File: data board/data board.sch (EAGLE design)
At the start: 41 parts, among them IC1 93LC56B, IC2 FT232HQ, U1 CJT1117-5.0-SOT223, X3 HUSB238, X6 USBC, Y1 12MHz

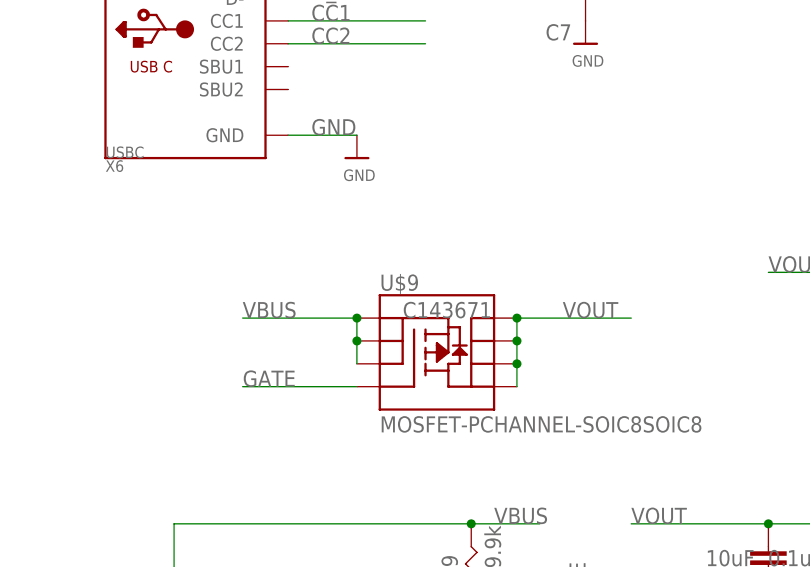
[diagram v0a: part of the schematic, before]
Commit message: v1.1
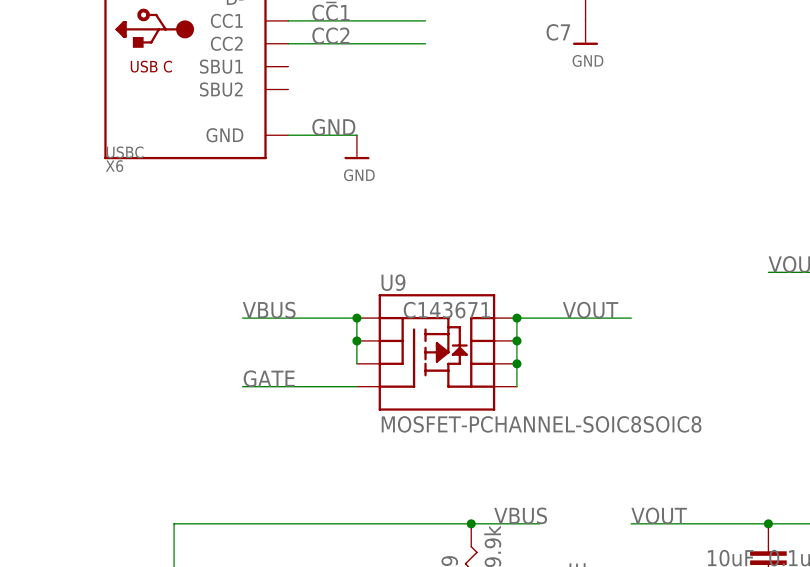
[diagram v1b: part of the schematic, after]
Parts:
- U1: LCSC (none) -> C89273
- renumbered U$9 to U9
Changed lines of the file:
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@@
 <part name="U$3" library="microbuilder" deviceset="GND" device=""/>
 <part name="JP3" library="microbuilder" deviceset="HEADER-1X3" device="ROUND"/>
-<part name="U1" library="Seeed-IC" library_urn="urn:adsk.eagle:library:470" deviceset="PMIC-CJT1117-5.0(SOT223)" device="" package3d_urn="urn:adsk.eagle:package:32638/1" value="CJT1117-5.0-SOT223"/>
+<part name="U1" library="Seeed-IC" library_urn="urn:adsk.eagle:library:470" deviceset="PMIC-CJT1117-5.0(SOT223)" device="" package3d_urn="urn:adsk.eagle:package:32638/1" value="CJT1117-5.0-SOT223">
+<attribute name="LCSC" value="C89273"/>
+</part>
 <part name="U$8" library="microbuilder" deviceset="GND" device=""/>
-<part name="U$9" library="SparkFun-DiscreteSemi" deviceset="MOSFET-PCHANNEL-SOIC8" device="SOIC8">
+<part name="U9" library="SparkFun-DiscreteSemi" deviceset="MOSFET-PCHANNEL-SOIC8" device="SOIC8">
 <attribute name="LCSC" value="C143671"/>
 </part>
@@
 <attribute name="NAME" x="307.34" y="135.89" size="1.27" layer="95"/>
 <attribute name="VALUE" x="314.96" y="135.89" size="1.27" layer="96"/>
+<attribute name="LCSC" x="314.96" y="132.08" size="1.778" layer="96" display="off"/>
 </instance>
 <instance part="U$8" gate="G$1" x="314.96" y="121.92" smashed="yes">
 <attribute name="VALUE" x="313.436" y="119.38" size="1.27" layer="96"/>
 </instance>
-<instance part="U$9" gate="G$1" x="248.92" y="124.46" smashed="yes">
+<instance part="U9" gate="G$1" x="248.92" y="124.46" smashed="yes">
 <attribute name="NAME" x="241.3" y="130.048" size="1.778" layer="95"/>
 <attribute name="VALUE" x="241.3" y="114.3" size="1.778" layer="96"/>
@@
 </segment>
 <segment>
-<pinref part="U$9" gate="G$1" pin="S@1"/>
+<pinref part="U9" gate="G$1" pin="S@1"/>
 <wire x1="238.76" y1="127" x2="226.06" y2="127" width="0.1524" layer="91"/>
-<pinref part="U$9" gate="G$1" pin="S@2"/>
+<pinref part="U9" gate="G$1" pin="S@2"/>
 <wire x1="238.76" y1="127" x2="238.76" y2="124.46" width="0.1524" layer="91"/>
 <junction x="238.76" y="127"/>
-<pinref part="U$9" gate="G$1" pin="S@3"/>
+<pinref part="U9" gate="G$1" pin="S@3"/>
 <wire x1="238.76" y1="124.46" x2="238.76" y2="121.92" width="0.1524" layer="91"/>
 <junction x="238.76" y="124.46"/>
@@
 </segment>
 <segment>
-<pinref part="U$9" gate="G$1" pin="D@4"/>
-<pinref part="U$9" gate="G$1" pin="D@3"/>
+<pinref part="U9" gate="G$1" pin="D@4"/>
+<pinref part="U9" gate="G$1" pin="D@3"/>
 <wire x1="256.54" y1="127" x2="256.54" y2="124.46" width="0.1524" layer="91"/>
-<pinref part="U$9" gate="G$1" pin="D@2"/>
+<pinref part="U9" gate="G$1" pin="D@2"/>
 <wire x1="256.54" y1="124.46" x2="256.54" y2="121.92" width="0.1524" layer="91"/>
 <junction x="256.54" y="124.46"/>
-<pinref part="U$9" gate="G$1" pin="D@1"/>
+<pinref part="U9" gate="G$1" pin="D@1"/>
 <wire x1="256.54" y1="121.92" x2="256.54" y2="119.38" width="0.1524" layer="91"/>
 <junction x="256.54" y="121.92"/>
@@
 </segment>
 <segment>
-<pinref part="U$9" gate="G$1" pin="G"/>
+<pinref part="U9" gate="G$1" pin="G"/>
 <wire x1="238.76" y1="119.38" x2="226.06" y2="119.38" width="0.1524" layer="91"/>
 <label x="226.06" y="119.38" size="1.778" layer="95"/>
